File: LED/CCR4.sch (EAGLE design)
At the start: 12 parts, among them Q2 STP11NM60ND, Q3 ST13003, X1 MKDSN1,5/2-5,08, X3 MKDSN1,5/2-5,08

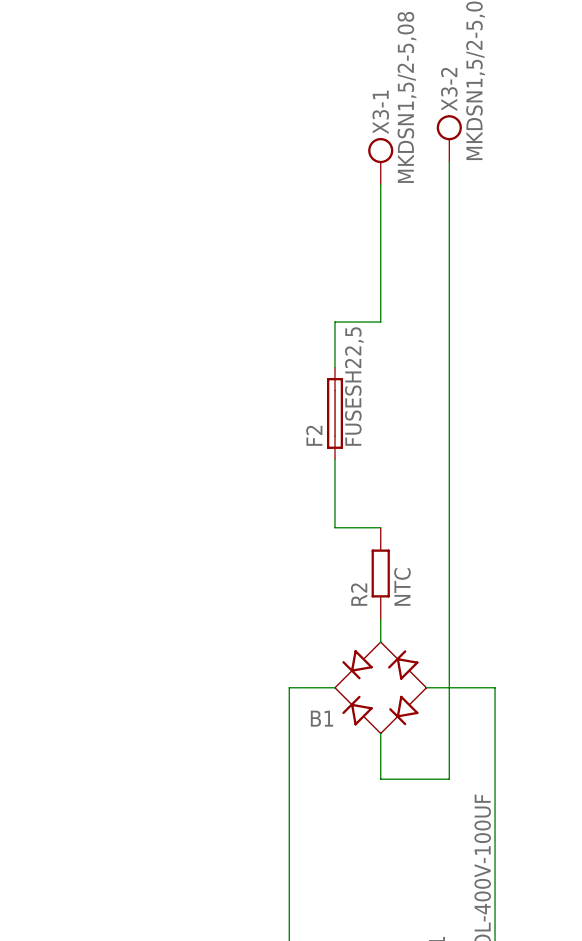
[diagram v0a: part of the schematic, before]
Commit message: _
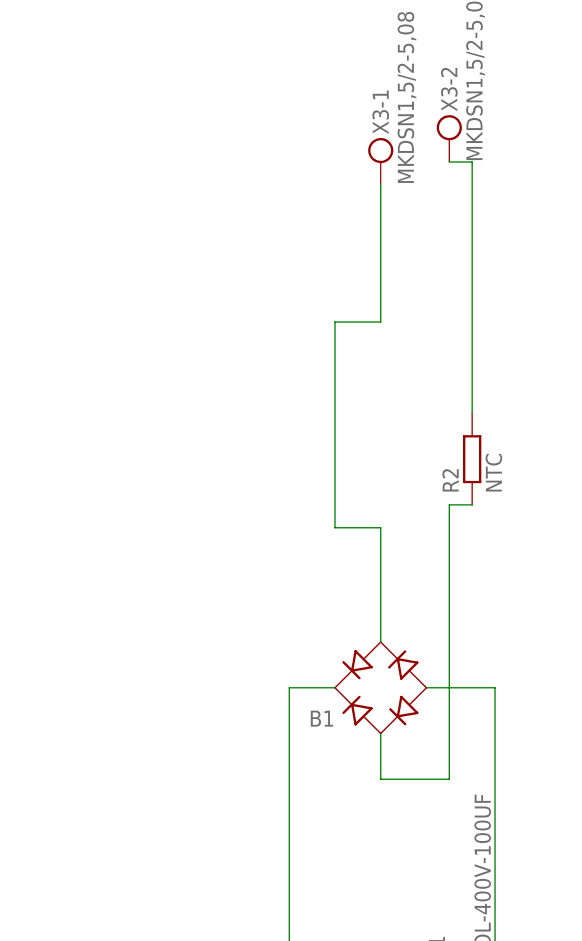
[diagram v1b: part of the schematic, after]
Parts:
- removed F2: FUSESH22,5, fuse:FUSESH22,5
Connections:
- removed net N$8: F2.1, R2.2
- net N$2: now also R2.1; no longer X3-2.KL
- net N$3: now also R2.2, X3-2.KL; no longer B1.AC2, R2.1
- net N$4: now also B1.AC2; no longer F2.2
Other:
- moved on the sheet: R2
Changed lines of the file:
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@@
 <part name="R2" library="rcl" deviceset="R-EU_" device="0309/10" value="NTC"/>
 <part name="U$1" library="Namenlos" deviceset="CPOL-400V-100UF" device=""/>
-<part name="F2" library="fuse" deviceset="FUSE" device="SH22,5"/>
 <part name="R4" library="rcl" deviceset="R-EU_" device="0411/12" value="13R"/>
 </parts>
@@
 <instance part="X3" gate="-1" x="68.58" y="193.04" rot="R90"/>
 <instance part="X3" gate="-2" x="76.2" y="195.58" rot="R90"/>
-<instance part="R2" gate="G$1" x="68.58" y="147.32" rot="R90"/>
+<instance part="R2" gate="G$1" x="78.74" y="160.02" rot="R90"/>
 <instance part="U$1" gate="G$1" x="77.47" y="101.6" rot="R90"/>
-<instance part="F2" gate="G$1" x="63.5" y="165.1" rot="R90"/>
 <instance part="R4" gate="G$1" x="20.32" y="35.56" rot="R90"/>
 </instances>
@@
 <segment>
 <pinref part="X3" gate="-1" pin="KL"/>
-<pinref part="F2" gate="G$1" pin="2"/>
 <wire x1="68.58" y1="175.26" x2="68.58" y2="190.5" width="0.1524" layer="91"/>
-<wire x1="63.5" y1="170.18" x2="63.5" y2="175.26" width="0.1524" layer="91"/>
 <wire x1="63.5" y1="175.26" x2="68.58" y2="175.26" width="0.1524" layer="91"/>
+<wire x1="63.5" y1="175.26" x2="63.5" y2="152.4" width="0.1524" layer="91"/>
+<pinref part="B1" gate="1" pin="AC2"/>
+<wire x1="63.5" y1="152.4" x2="68.58" y2="152.4" width="0.1524" layer="91"/>
+<wire x1="68.58" y1="152.4" x2="68.58" y2="139.7" width="0.1524" layer="91"/>
 </segment>
 </net>
@@
 <wire x1="68.58" y1="129.54" x2="68.58" y2="124.46" width="0.1524" layer="91"/>
 <wire x1="68.58" y1="124.46" x2="76.2" y2="124.46" width="0.1524" layer="91"/>
-<pinref part="X3" gate="-2" pin="KL"/>
-<wire x1="76.2" y1="193.04" x2="76.2" y2="124.46" width="0.1524" layer="91"/>
-</segment>
-</net>
-<net name="N$8" class="0">
-<segment>
-<pinref part="F2" gate="G$1" pin="1"/>
-<wire x1="63.5" y1="160.02" x2="63.5" y2="152.4" width="0.1524" layer="91"/>
-<wire x1="63.5" y1="152.4" x2="68.58" y2="152.4" width="0.1524" layer="91"/>
-<pinref part="R2" gate="G$1" pin="2"/>
+<pinref part="R2" gate="G$1" pin="1"/>
+<wire x1="78.74" y1="154.94" x2="76.2" y2="154.94" width="0.1524" layer="91"/>
+<wire x1="76.2" y1="154.94" x2="76.2" y2="124.46" width="0.1524" layer="91"/>
 </segment>
 </net>
 <net name="N$3" class="0">
 <segment>
-<pinref part="R2" gate="G$1" pin="1"/>
-<pinref part="B1" gate="1" pin="AC2"/>
-<wire x1="68.58" y1="142.24" x2="68.58" y2="139.7" width="0.1524" layer="91"/>
+<pinref part="X3" gate="-2" pin="KL"/>
+<pinref part="R2" gate="G$1" pin="2"/>
+<wire x1="76.2" y1="193.04" x2="78.74" y2="193.04" width="0.1524" layer="91"/>
+<wire x1="78.74" y1="193.04" x2="78.74" y2="165.1" width="0.1524" layer="91"/>
 </segment>
 </net>
